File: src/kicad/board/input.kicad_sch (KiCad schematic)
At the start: 19 parts, among them SW1 SW_Keyboard, SW2 SW_Keyboard, SW3 RotEncoder_S, SW4 SW_Keyboard, SW5 SW_Keyboard, U5 74HC4051, U6 4072

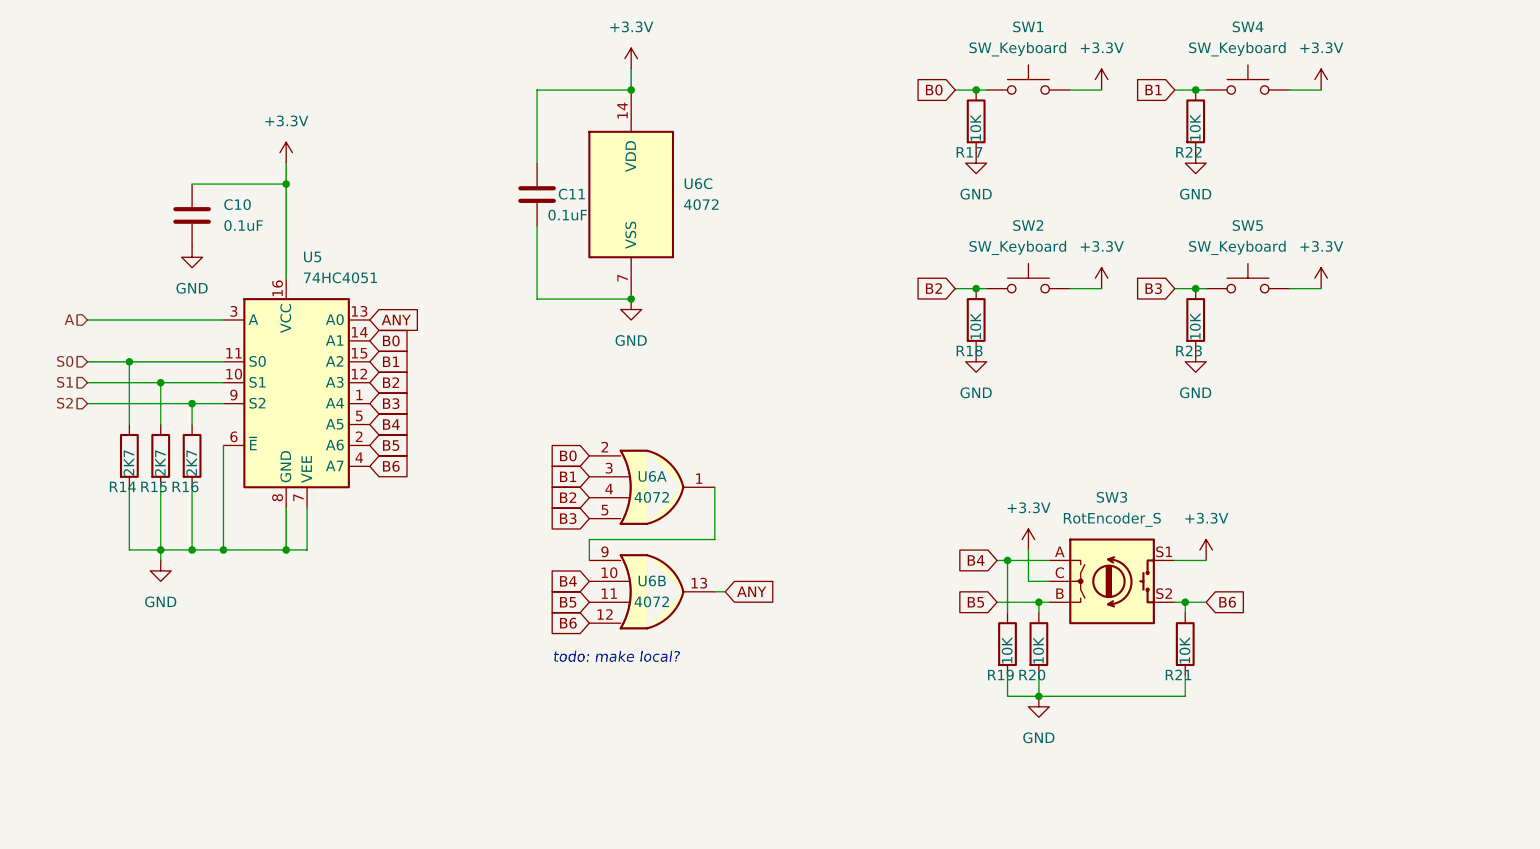
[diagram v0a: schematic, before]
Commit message: update
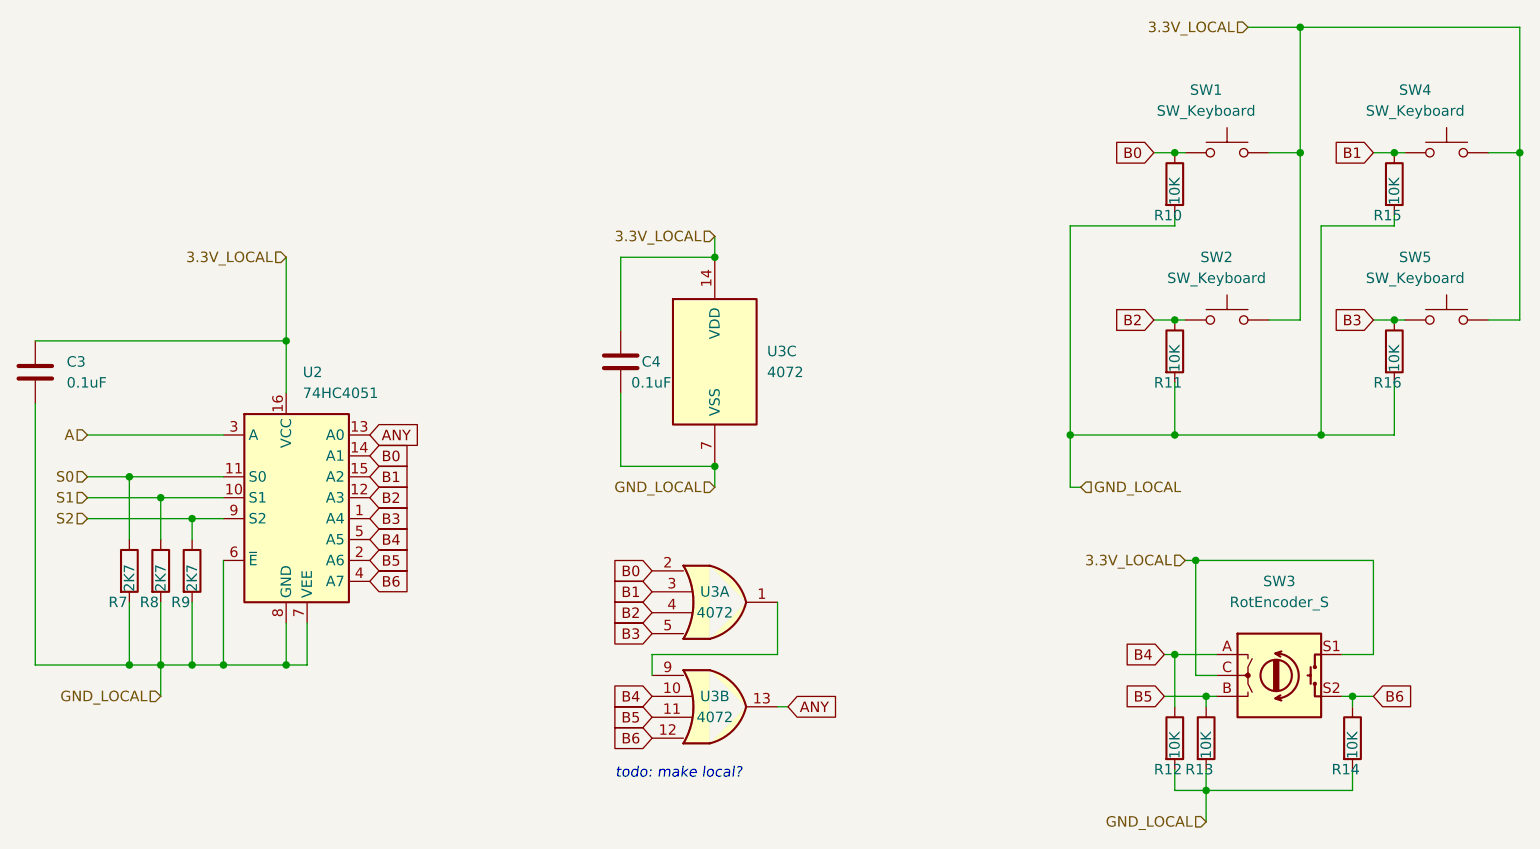
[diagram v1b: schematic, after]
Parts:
- renumbered C10 to C3, C11 to C4, R17 to R10, R18 to R11, R19 to R12, R20 to R13, R21 to R14, R22 to R15, R23 to R16, R14 to R7, R15 to R8, R16 to R9, U5 to U2, U6 to U3
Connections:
- net +3.3V renamed 3.3V_LOCAL
- net GND renamed GND_LOCAL
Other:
- moved on the sheet: C3, C4, R10, R11, R12, R13, R14, R15, R16, R7, R8, R9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
